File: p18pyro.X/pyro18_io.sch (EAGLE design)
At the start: 2 parts, among them X2 332-10

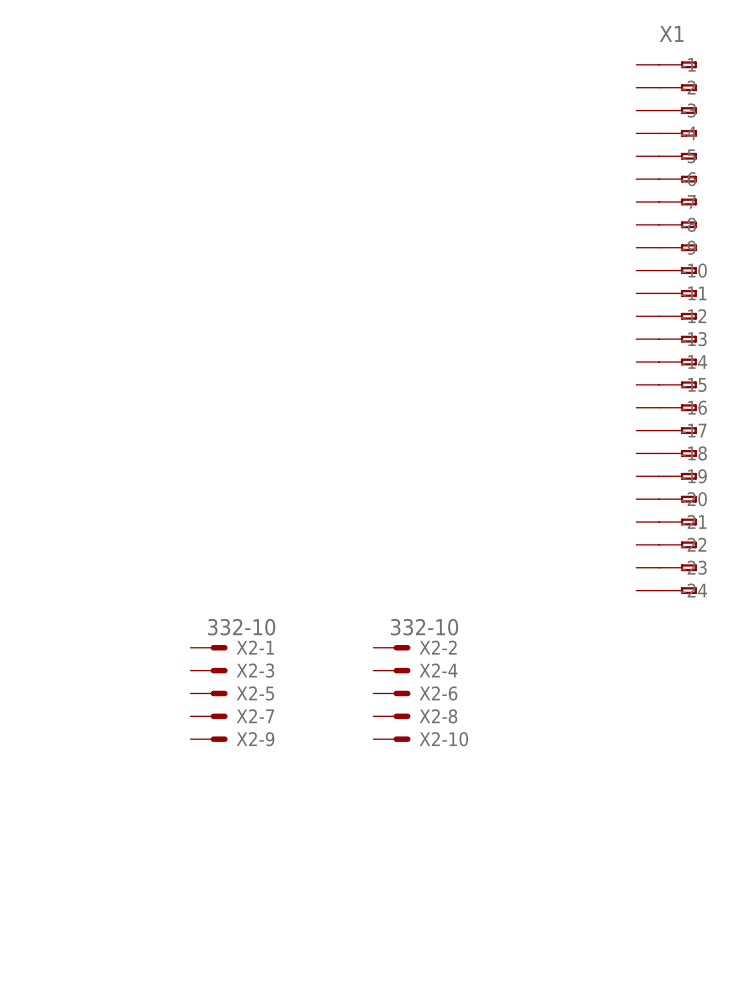
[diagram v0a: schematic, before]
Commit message: update
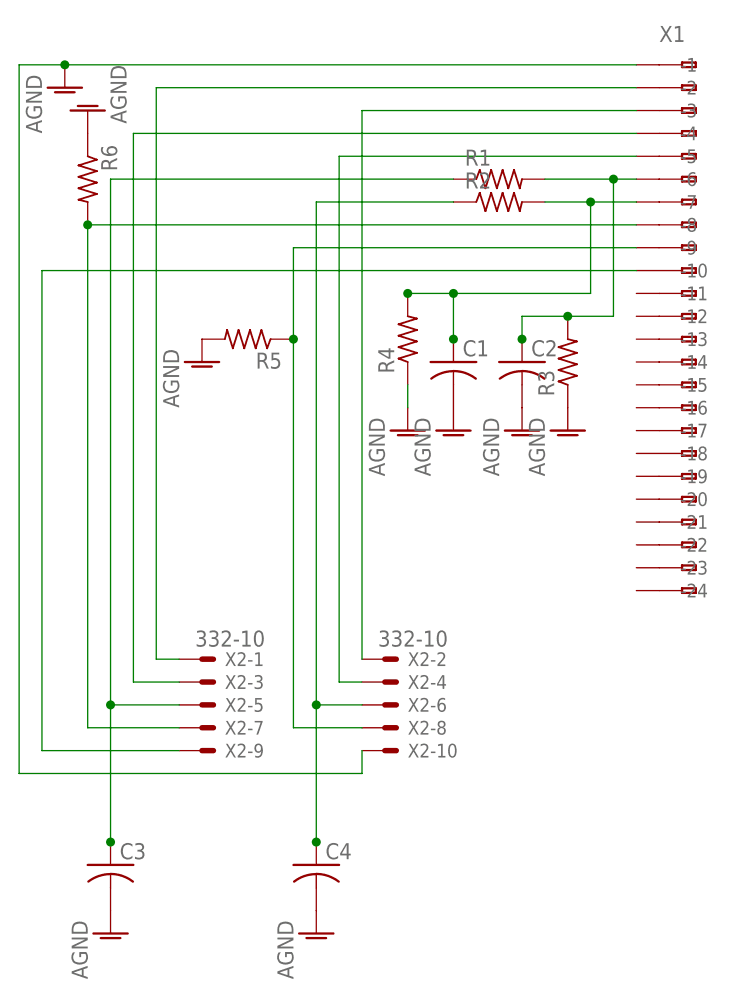
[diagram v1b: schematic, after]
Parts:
- added C1, C2, C3, C4: (no value), resistor:C-US025-024X044
- added R1, R2, R3, R4, R5, R6: (no value), resistor:R-US_0204/2V
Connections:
- new net AGND: C1.2, C2.2, C3.2, C4.2, R3.1, R4.1, R5.2, R6.1, X1.-1, X2-10.S
- new net N$1: C1.1, R2.2, R4.2, X1.-7
- new net N$10: R5.1, X1.-9, X2-8.S
- new net N$11: C2.1, R1.2, R3.2, X1.-6
- new net N$2: X1.-10, X2-9.S
- new net N$3: X1.-4, X2-3.S
- new net N$4: X1.-2, X2-1.S
- new net N$5: X1.-3, X2-2.S
- new net N$6: X1.-5, X2-4.S
- new net N$7: C3.1, R1.1, X2-5.S
- new net N$8: C4.1, R2.1, X2-6.S
- new net N$9: R6.2, X1.-8, X2-7.S
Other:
- moved on the sheet: X2-1, X2-10, X2-2, X2-3, X2-4, X2-5, X2-6, X2-7, X2-8, X2-9
